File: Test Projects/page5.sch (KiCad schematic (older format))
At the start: 21 parts, among them P21 CONN_01X07, U13 SF-4052, U14 SF-4052, U15 SF-4052, U16 SF-4052, U17 SF-4052, U18 SF-4052, U19 SF-4052, U20 SF-4052, U21 SF-4052, U22 SF-4052

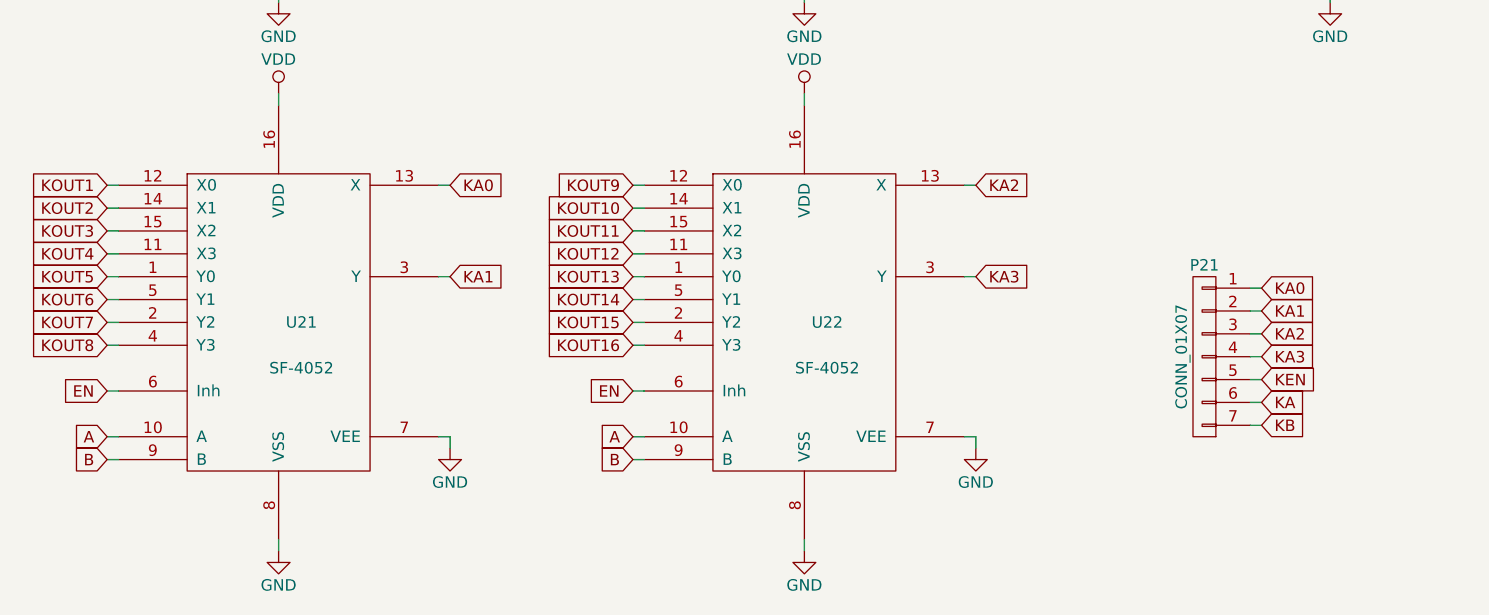
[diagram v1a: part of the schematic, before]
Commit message: more layout
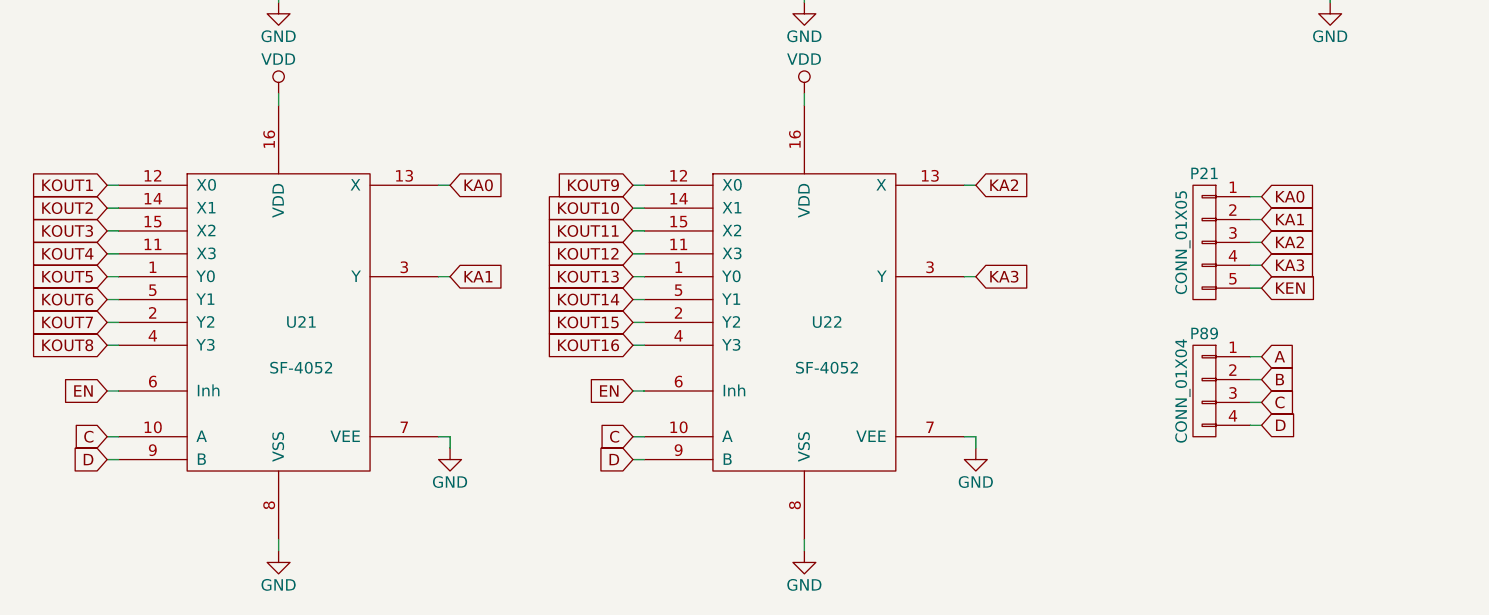
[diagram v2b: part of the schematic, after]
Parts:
- removed P21: CONN_01X07, Pin_Headers:Pin_Header_Straight_1x07, symbol CONN_01X07
- added P21: CONN_01X05, Pin_Headers:Pin_Header_Straight_1x05, symbol CONN_01X05
- added P89: CONN_01X04, Pin_Headers:Pin_Header_Straight_1x04, symbol CONN_01X04
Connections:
- net A: now also P89.1 (P1); no longer U21.10 (A), U22.10 (A)
- net B: now also P89.2 (P2); no longer U21.9 (B), U22.9 (B)
- net KA0: now also P21.1 (P1)
- net KA1: now also P21.2 (P2)
- net KA2: now also P21.3 (P3)
- net KA3: now also P21.4 (P4)
- net KEN: now also P21.5 (P5)
- new net C: P89.3 (P3), U21.10 (A), U22.10 (A)
- new net D: P89.4 (P4), U21.9 (B), U22.9 (B)
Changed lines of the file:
@@
 LIBS:SparkFun-Mounting
 LIBS:SparkFun-Opto
+LIBS:SparkFun-Connectors
 LIBS:Teensy_test_layout-cache
 EELAYER 25 0
@@
 	3350 2350 3400 2350
 Text GLabel 1050 7100 0    50   Input ~ 0
-A
+C
 Text GLabel 1050 7200 0    50   Input ~ 0
-B
+D
 Wire Wire Line
 	1100 7100 1050 7100
 Wire Wire Line
 	1050 7200 1100 7200
-Text GLabel 6100 6650 2    50   Input ~ 0
+Text GLabel 6100 6250 2    50   Input ~ 0
 KA2
-Text GLabel 6100 6750 2    50   Input ~ 0
+Text GLabel 6100 6350 2    50   Input ~ 0
 KA3
 $Comp
@@
 Wire Wire Line
 	1050 2050 1100 2050
+Text GLabel 6100 6450 2    50   Input ~ 0
+KEN
+Text GLabel 6100 6750 2    50   Input ~ 0
+A
 Text GLabel 6100 6850 2    50   Input ~ 0
-KEN
-Text GLabel 6100 6950 2    50   Input ~ 0
-KA
-Text GLabel 6100 7050 2    50   Input ~ 0
-KB
-$Comp
-L CONN_01X07 P21
-U 1 1 5688BBDD
-P 5850 6750
-F 0 "P21" H 5850 7150 50  0000 C CNN
-F 1 "CONN_01X07" V 5950 6750 50  0000 C CNN
-F 2 "Pin_Headers:Pin_Header_Straight_1x07" H 5850 6750 50  0001 C CNN
-F 3 "" H 5850 6750 50  0000 C CNN
-	1    5850 6750
-	-1   0    0    -1
-$EndComp
-Wire Wire Line
-	6050 6650 6100 6650
+B
+Wire Wire Line
+	6050 6250 6100 6250
+Wire Wire Line
+	6100 6350 6050 6350
+Wire Wire Line
+	6050 6450 6100 6450
 Wire Wire Line
 	6100 6750 6050 6750
 Wire Wire Line
 	6050 6850 6100 6850
-Wire Wire Line
-	6100 6950 6050 6950
-Wire Wire Line
-	6050 7050 6100 7050
 $Comp
 L C C24
@@
 	3350 4800 3400 4800
 Text GLabel 3350 7100 0    50   Input ~ 0
-A
+C
 Text GLabel 3350 7200 0    50   Input ~ 0
-B
+D
 Wire Wire Line
 	3400 7100 3350 7100
@@
 Text GLabel 5650 4300 0    50   Input ~ 0
 K56
-Text GLabel 6100 6550 2    50   Input ~ 0
+Text GLabel 6100 6150 2    50   Input ~ 0
 KA1
-Text GLabel 6100 6450 2    50   Input ~ 0
+Text GLabel 6100 6050 2    50   Input ~ 0
 KA0
 Wire Wire Line
-	6050 6550 6100 6550
-Wire Wire Line
-	6100 6450 6050 6450
+	6050 6150 6100 6150
+Wire Wire Line
+	6100 6050 6050 6050
 $Comp
 L SF-4052 U13
@@
 Wire Wire Line
 	8700 3200 8700 3250
+$Comp
+L CONN_01X04 P89
+U 1 1 56AAE984
+P 5850 6900
+F 0 "P89" H 5850 7150 50  0000 C CNN
+F 1 "CONN_01X04" V 5950 6900 50  0000 C CNN
+F 2 "Pin_Headers:Pin_Header_Straight_1x04" H 5850 6900 50  0001 C CNN
+F 3 "" H 5850 6900 50  0000 C CNN
+	1    5850 6900
+	-1   0    0    -1
+$EndComp
+$Comp
+L CONN_01X05 P21
+U 1 1 56AAE9F7
+P 5850 6250
+F 0 "P21" H 5850 6550 50  0000 C CNN
+F 1 "CONN_01X05" V 5950 6250 50  0000 C CNN
+F 2 "Pin_Headers:Pin_Header_Straight_1x05" H 5850 6250 50  0001 C CNN
+F 3 "" H 5850 6250 50  0000 C CNN
+	1    5850 6250
+	-1   0    0    -1
+$EndComp
+Text GLabel 6100 7050 2    50   Input ~ 0
+D
+Wire Wire Line
+	6050 7050 6100 7050
+Text GLabel 6100 6950 2    50   Input ~ 0
+C
+Wire Wire Line
+	6050 6950 6100 6950
 $EndSCHEMATC
